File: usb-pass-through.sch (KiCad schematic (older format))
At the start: 7 parts, among them P6 USB_B, P9 USB_A

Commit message: Update with kicad-helpers files
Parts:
- C39: symbol C_Small -> Device:C_Small
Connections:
- wire segments 30 -> 36
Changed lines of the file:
@@
-EESchema Schematic File Version 2
-LIBS:power
-LIBS:device
-LIBS:transistors
-LIBS:conn
-LIBS:linear
-LIBS:regul
-LIBS:74xx
-LIBS:cmos4000
-LIBS:adc-dac
-LIBS:memory
-LIBS:xilinx
-LIBS:microcontrollers
-LIBS:dsp
-LIBS:microchip
-LIBS:analog_switches
-LIBS:motorola
-LIBS:texas
-LIBS:intel
-LIBS:audio
-LIBS:interface
-LIBS:digital-audio
-LIBS:philips
-LIBS:display
-LIBS:cypress
-LIBS:siliconi
-LIBS:opto
-LIBS:atmel
-LIBS:contrib
-LIBS:valves
-LIBS:sci-bots
-LIBS:dropbot_control_board-cache
-EELAYER 25 0
+EESchema Schematic File Version 4
+EELAYER 30 0
 EELAYER END
 $Descr USLetter 11000 8500
@@
 	4850 3450 4750 3450
 Wire Wire Line
-	4750 3250 4750 4150
+	4750 3250 4750 3450
 Wire Wire Line
 	4750 3850 4850 3850
 Connection ~ 4750 3450
 Wire Wire Line
-	5550 3250 5550 4150
+	5550 3250 5550 3450
 Wire Wire Line
 	5550 3850 5450 3850
@@
 $EndComp
 Wire Wire Line
-	4550 3200 4550 3900
+	4550 3200 4550 3650
 $Comp
 L FERRITE FB8
@@
 $EndComp
 Wire Wire Line
-	4550 4200 4550 4400
-$Comp
-L C_Small C39
+	4550 4200 4550 4300
+$Comp
+L Device:C_Small C39
 U 1 1 58BE5178
 P 4250 4300
@@
 	5700 4700 5400 4700
 $Comp
-L GND #PWR025
+L power:GND #PWR025
 U 1 1 5B3C7E87
 P 4800 5100
@@
 	1    0    0    -1
 $EndComp
+Wire Wire Line
+	4750 3450 4750 3850
+Wire Wire Line
+	5550 3450 5550 3850
+Wire Wire Line
+	4750 3850 4750 4150
+Wire Wire Line
+	5550 3850 5550 4150
+Wire Wire Line
+	4550 4300 4550 4400
+Wire Wire Line
+	4550 3650 4550 3900
 $EndSCHEMATC

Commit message: Fix broken symbols and DRC tests
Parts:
- D5: symbol WE-TVS_824015 -> sci-bots:WE-TVS_824015
- FB7, FB8: symbol FERRITE -> sci-bots:FERRITE
- L2: symbol CM_CHOKE -> sci-bots:CM_CHOKE
- P6: symbol USB_B -> Connector:USB_B
- P9: symbol USB_A -> Connector:USB_A
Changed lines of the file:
@@
 CHASIS_GND
 $Comp
-L WE-TVS_824015 D5
+L sci-bots:WE-TVS_824015 D5
 U 1 1 58BAFF99
 P 5150 3650
@@
 $EndComp
 $Comp
-L CM_CHOKE L2
+L sci-bots:CM_CHOKE L2
 U 1 1 58BBE1AE
 P 5150 4300
@@
 	5200 4150 5200 4200
 $Comp
-L FERRITE FB7
+L sci-bots:FERRITE FB7
 U 1 1 58BE3979
 P 4550 4050
@@
 	4550 3200 4550 3650
 $Comp
-L FERRITE FB8
+L sci-bots:FERRITE FB8
 U 1 1 58BE422E
 P 4550 4550
@@
 Wire Wire Line
 	4850 3650 4550 3650
-Text GLabel 5200 4550 2    60   Input ~ 0
-D+
-Text GLabel 5100 4550 0    60   Input ~ 0
-D-
 Wire Wire Line
 	4350 4300 4550 4300
@@
 	3950 4300 4150 4300
 $Comp
-L USB_B P6
+L Connector:USB_B P6
 U 1 1 59320548
 P 5200 2800
@@
 	5700 3650 5450 3650
 $Comp
-L USB_A P9
+L Connector:USB_A P9
 U 1 1 59320AF4
 P 5200 5000
@@
 Wire Wire Line
 	4550 3650 4550 3900
+Text Label 5100 4600 2    60   ~ 0
+D-
+Text Label 5200 4600 0    60   ~ 0
+D+
+$Comp
+L power:PWR_FLAG #FLG0104
+U 1 1 61967CD9
+P 4550 5300
+F 0 "#FLG0104" H 4550 5375 50  0001 C CNN
+F 1 "PWR_FLAG" H 4550 5473 50  0000 C CNN
+F 2 "" H 4550 5300 50  0001 C CNN
+F 3 "~" H 4550 5300 50  0001 C CNN
+	1    4550 5300
+	-1   0    0    1
+$EndComp
+Connection ~ 4550 5300
 $EndSCHEMATC

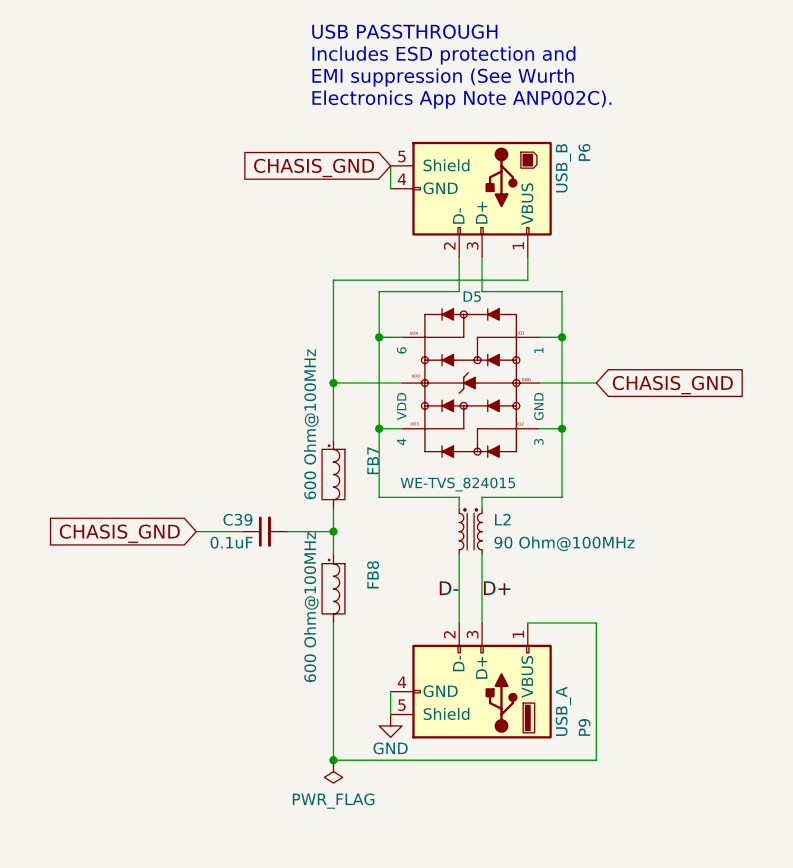
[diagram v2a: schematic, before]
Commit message: Update BOM
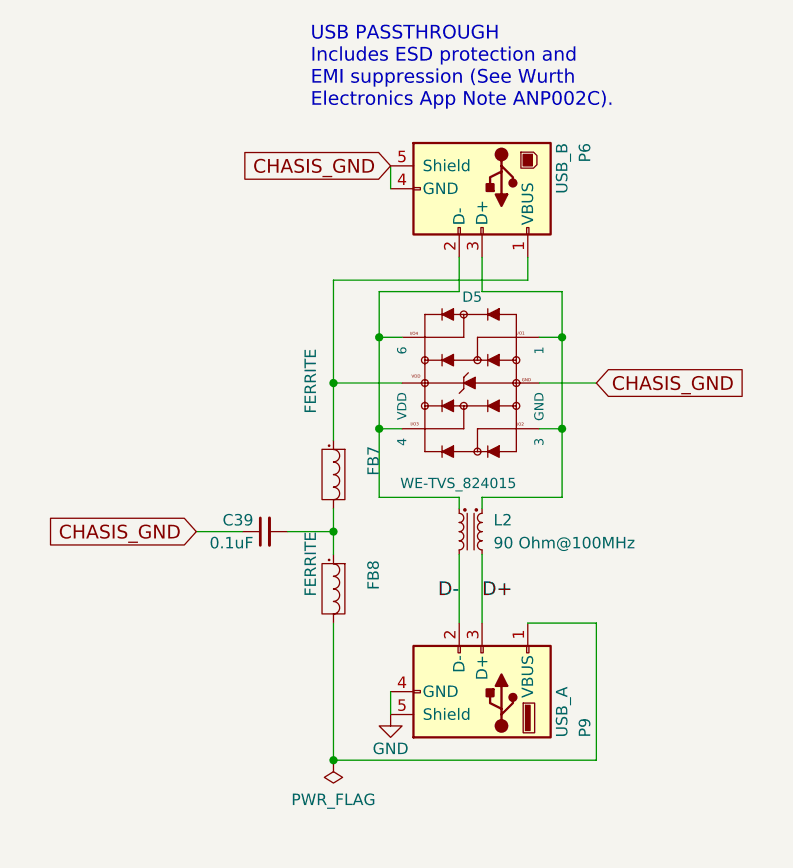
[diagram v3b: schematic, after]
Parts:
- C39: MPN (none) -> CL21B104KBCNNNC; Manufacturer (none) -> Samsung
- D5: MPN (none) -> 824015; Manufacturer (none) -> Würth Elektronik
- FB7, FB8: value 600 Ohm@100MHz -> FERRITE; MPN (none) -> 742792040; Manufacturer (none) -> Würth Elektronik
- L2: MPN (none) -> 744231091; Manufacturer (none) -> Würth Elektronik
- P6: MPN (none) -> 1734346-1; Manufacturer (none) -> TE Connectivity
- P9: MPN (none) -> AU-Y1006; Manufacturer (none) -> ASSMANN WSW Components
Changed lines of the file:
@@
 Comment4 ""
 $EndDescr
+$Comp
+L sci-bots:WE-TVS_824015 D5
+U 1 1 58BAFF99
+P 5150 3650
+F 0 "D5" V 4800 3600 45 0000 L BNN
+F 1 "WE-TVS_824015" V 5615 3450 45 0000 L BNN
+F 2 "Sci-Bots:wurth-WE-TVS_SOT23-6L" H 5180 3800 20 0001 C CNN
+F 3 "" H 5150 3650 60 0000 C CNN
+F 4 "824015" H 4800 3700 50 0001 C CNN "MPN"
+F 5 "Würth Elektronik" H 4800 3700 50 0001 C CNN "Manufacturer"
+F 6 "824015" H 5150 3650 60 0001 C CNN "Mfg_Part_No"
+	1    5150 3650
+	0    -1   1    0
+$EndComp
+$Comp
+L sci-bots:CM_CHOKE L2
+U 1 1 58BBE1AE
+P 5150 4300
+F 0 "L2" H 5250 4350 50 0000 L CNN
+F 1 "90 Ohm@100MHz" H 5250 4250 50 0000 L CNN
+F 2 "Sci-Bots:wurth-WE-CNSW_0805" H 5200 4300 50 0001 C CNN
+F 3 "" H 5200 4300 50 0000 C CNN
+F 4 "744231091" H 5250 4450 50 0001 C CNN "MPN"
+F 5 "Würth Elektronik" H 5250 4450 50 0001 C CNN "Manufacturer"
+F 6 "744231091" H 5150 4300 60 0001 C CNN "Mfg_Part_No"
+	1    5150 4300
+	1    0    0    -1
+$EndComp
+$Comp
+L sci-bots:FERRITE FB7
+U 1 1 58BE3979
+P 4550 4050
+F 0 "FB7" H 4425 4225 50 0000 L CNN
+F 1 "FERRITE" H 4000 3950 50 0000 L CNN
+F 2 "Resistors_SMD:R_0805" H 4550 3950 60 0001 C CNN
+F 3 "" H 4550 3950 60 0000 C CNN
+F 4 "742792040" H 4425 4325 50 0001 C CNN "MPN"
+F 5 "Würth Elektronik" H 4425 4325 50 0001 C CNN "Manufacturer"
+F 6 "742792040" H 4550 4050 60 0001 C CNN "Mfg_Part_No"
+	1    4550 4050
+	0    1    1    0
+$EndComp
+$Comp
+L sci-bots:FERRITE FB8
+U 1 1 58BE422E
+P 4550 4550
+F 0 "FB8" H 4425 4725 50 0000 L CNN
+F 1 "FERRITE" H 4300 4450 50 0000 L CNN
+F 2 "Resistors_SMD:R_0805" H 4550 4450 60 0001 C CNN
+F 3 "" H 4550 4450 60 0000 C CNN
+F 4 "742792040" H 4425 4825 50 0001 C CNN "MPN"
+F 5 "Würth Elektronik" H 4425 4825 50 0001 C CNN "Manufacturer"
+F 6 "742792040" H 4550 4550 60 0001 C CNN "Mfg_Part_No"
+	1    4550 4550
+	0    1    1    0
+$EndComp
+$Comp
+L Device:C_Small C39
+U 1 1 58BE5178
+P 4250 4300
+F 0 "C39" V 4300 4350 50 0000 L CNN
+F 1 "0.1uF" V 4200 4350 50 0000 L CNN
+F 2 "Capacitors_SMD:C_0805" H 4250 4300 50 0001 C CNN
+F 3 "" H 4250 4300 50 0000 C CNN
+F 4 "CL21B104KBCNNNC" H 4300 4450 50 0001 C CNN "MPN"
+F 5 "Samsung" H 4300 4450 50 0001 C CNN "Manufacturer"
+F 6 "CL21B104KBCNNNC" H 4250 4300 60 0001 C CNN "Mfg_Part_No"
+	1    4250 4300
+	0    -1   -1   0
+$EndComp
+$Comp
+L Connector:USB_B P6
+U 1 1 59320548
+P 5200 2800
+F 0 "P6" H 5000 3250 50 0000 L CNN
+F 1 "USB_B" H 5000 3150 50 0000 L CNN
+F 2 "Sci-Bots:1734346-1" H 5350 2750 50 0001 C CNN
+F 3 "" H 5350 2750 50 0001 C CNN
+F 4 "1734346-1" H 5000 3350 50 0001 C CNN "MPN"
+F 5 "TE Connectivity" H 5000 3350 50 0001 C CNN "Manufacturer"
+F 6 "1734346-1" H 5200 2800 60 0001 C CNN "Mfg_Part_No"
+	1    5200 2800
+	0    1    1    0
+$EndComp
+$Comp
+L Connector:USB_A P9
+U 1 1 59320AF4
+P 5200 5000
+F 0 "P9" H 5000 5450 50 0000 L CNN
+F 1 "USB_A" H 5000 5350 50 0000 L CNN
+F 2 "Sci-Bots:AU-Y1006" H 5350 4950 50 0001 C CNN
+F 3 "" H 5350 4950 50 0001 C CNN
+F 4 "AU-Y1006" H 5000 5550 50 0001 C CNN "MPN"
+F 5 "ASSMANN WSW Components" H 5000 5550 50 0001 C CNN "Manufacturer"
+F 6 "AU-Y1006" H 5200 5000 60 0001 C CNN "Mfg_Part_No"
+	1    5200 5000
+	0    1    -1   0
+$EndComp
+$Comp
+L power:GND #PWR025
+U 1 1 5B3C7E87
+P 4800 5100
+F 0 "#PWR025" H 4800 4850 50 0001 C CNN
+F 1 "GND" H 4800 4950 50 0000 C CNN
+F 2 "" H 4800 5100 50 0001 C CNN
+F 3 "" H 4800 5100 50 0001 C CNN
+	1    4800 5100
+	1    0    0    -1
+$EndComp
+$Comp
+L power:PWR_FLAG #FLG0104
+U 1 1 61967CD9
+P 4550 5300
+F 0 "#FLG0104" H 4550 5375 50 0001 C CNN
+F 1 "PWR_FLAG" H 4550 5473 50 0000 C CNN
+F 2 "" H 4550 5300 50 0001 C CNN
+F 3 "~" H 4550 5300 50 0001 C CNN
+	1    4550 5300
+	-1   0    0    1
+$EndComp
 Text Notes 4450 2450 0    60   ~ 0
 USB PASSTHROUGH\nIncludes ESD protection and\nEMI suppression (See Wurth\nElectronics App Note ANP002C).
 Text GLabel 5700 3650 2    60   Input ~ 0
 CHASIS_GND
-$Comp
-L sci-bots:WE-TVS_824015 D5
-U 1 1 58BAFF99
-P 5150 3650
-F 0 "D5" V 4800 3600 45  0000 L BNN
-F 1 "WE-TVS_824015" V 5615 3450 45  0000 L BNN
-F 2 "Sci-Bots:wurth-WE-TVS_SOT23-6L" H 5180 3800 20  0001 C CNN
-F 3 "" H 5150 3650 60  0000 C CNN
-F 4 "824015" H 5150 3650 60  0001 C CNN "Mfg_Part_No"
-	1    5150 3650
-	0    -1   1    0
-$EndComp
-$Comp
-L sci-bots:CM_CHOKE L2
-U 1 1 58BBE1AE
-P 5150 4300
-F 0 "L2" H 5250 4350 50  0000 L CNN
-F 1 "90 Ohm@100MHz" H 5250 4250 50  0000 L CNN
-F 2 "Sci-Bots:wurth-WE-CNSW_0805" H 5200 4300 50  0001 C CNN
-F 3 "" H 5200 4300 50  0000 C CNN
-F 4 "744231091" H 5150 4300 60  0001 C CNN "Mfg_Part_No"
-	1    5150 4300
-	1    0    0    -1
-$EndComp
-Wire Wire Line
-	5100 3100 5100 3250
-Wire Wire Line
-	5100 3250 4750 3250
-Wire Wire Line
-	5200 3100 5200 3250
-Wire Wire Line
-	5200 3250 5550 3250
-Wire Wire Line
-	4850 3450 4750 3450
-Wire Wire Line
-	4750 3250 4750 3450
-Wire Wire Line
-	4750 3850 4850 3850
-Connection ~ 4750 3450
-Wire Wire Line
-	5550 3250 5550 3450
-Wire Wire Line
-	5550 3850 5450 3850
-Wire Wire Line
-	5450 3450 5550 3450
-Connection ~ 5550 3450
-Connection ~ 4750 3850
-Connection ~ 5550 3850
-Wire Wire Line
-	4750 4150 5100 4150
-Wire Wire Line
-	5550 4150 5200 4150
-Wire Wire Line
-	5100 4150 5100 4200
-Wire Wire Line
-	5200 4150 5200 4200
-$Comp
-L sci-bots:FERRITE FB7
-U 1 1 58BE3979
-P 4550 4050
-F 0 "FB7" H 4425 4225 50  0000 L CNN
-F 1 "600 Ohm@100MHz" H 4000 3950 50  0000 L CNN
-F 2 "Resistors_SMD:R_0805" H 4550 3950 60  0001 C CNN
-F 3 "" H 4550 3950 60  0000 C CNN
-F 4 "742792040" H 4550 4050 60  0001 C CNN "Mfg_Part_No"
-	1    4550 4050
-	0    1    1    0
-$EndComp
-Wire Wire Line
-	4550 3200 4550 3650
-$Comp
-L sci-bots:FERRITE FB8
-U 1 1 58BE422E
-P 4550 4550
-F 0 "FB8" H 4425 4725 50  0000 L CNN
-F 1 "600 Ohm@100MHz" H 4300 4450 50  0000 L CNN
-F 2 "Resistors_SMD:R_0805" H 4550 4450 60  0001 C CNN
-F 3 "" H 4550 4450 60  0000 C CNN
-F 4 "742792040" H 4550 4550 60  0001 C CNN "Mfg_Part_No"
-	1    4550 4550
-	0    1    1    0
-$EndComp
-Wire Wire Line
-	4550 4200 4550 4300
-$Comp
-L Device:C_Small C39
-U 1 1 58BE5178
-P 4250 4300
-F 0 "C39" V 4300 4350 50  0000 L CNN
-F 1 "0.1uF" V 4200 4350 50  0000 L CNN
-F 2 "Capacitors_SMD:C_0805" H 4250 4300 50  0001 C CNN
-F 3 "" H 4250 4300 50  0000 C CNN
-F 4 "CL21B104KBCNNNC" H 4250 4300 60  0001 C CNN "Mfg_Part_No"
-	1    4250 4300
-	0    -1   -1   0
-$EndComp
-Connection ~ 4550 4300
-Connection ~ 4550 3650
-Wire Wire Line
-	4850 3650 4550 3650
-Wire Wire Line
-	4350 4300 4550 4300
 Text GLabel 3950 4300 0    60   Input ~ 0
 CHASIS_GND
-Wire Wire Line
-	3950 4300 4150 4300
-$Comp
-L Connector:USB_B P6
-U 1 1 59320548
-P 5200 2800
-F 0 "P6" H 5000 3250 50  0000 L CNN
-F 1 "USB_B" H 5000 3150 50  0000 L CNN
-F 2 "Sci-Bots:1734346-1" H 5350 2750 50  0001 C CNN
-F 3 "" H 5350 2750 50  0001 C CNN
-F 4 "1734346-1" H 5200 2800 60  0001 C CNN "Mfg_Part_No"
-	1    5200 2800
-	0    1    1    0
-$EndComp
-Wire Wire Line
-	4550 3200 5400 3200
-Wire Wire Line
-	5400 3200 5400 3100
-Wire Wire Line
-	5700 3650 5450 3650
-$Comp
-L Connector:USB_A P9
-U 1 1 59320AF4
-P 5200 5000
-F 0 "P9" H 5000 5450 50  0000 L CNN
-F 1 "USB_A" H 5000 5350 50  0000 L CNN
-F 2 "Sci-Bots:AU-Y1006" H 5350 4950 50  0001 C CNN
-F 3 "" H 5350 4950 50  0001 C CNN
-F 4 "AU-Y1006" H 5200 5000 60  0001 C CNN "Mfg_Part_No"
-	1    5200 5000
-	0    1    -1   0
-$EndComp
 Text GLabel 4800 2700 0    60   Input ~ 0
 CHASIS_GND
-Wire Wire Line
-	4800 2800 4800 2700
-Wire Wire Line
-	5100 4700 5100 4400
-Wire Wire Line
-	5200 4400 5200 4700
-Wire Wire Line
-	4800 5000 4800 5100
-Wire Wire Line
-	4550 4700 4550 5300
-Wire Wire Line
-	4550 5300 5700 5300
-Wire Wire Line
-	5700 5300 5700 4700
-Wire Wire Line
-	5700 4700 5400 4700
-$Comp
-L power:GND #PWR025
-U 1 1 5B3C7E87
-P 4800 5100
-F 0 "#PWR025" H 4800 4850 50  0001 C CNN
-F 1 "GND" H 4800 4950 50  0000 C CNN
-F 2 "" H 4800 5100 50  0001 C CNN
-F 3 "" H 4800 5100 50  0001 C CNN
-	1    4800 5100
-	1    0    0    -1
-$EndComp
-Wire Wire Line
-	4750 3450 4750 3850
-Wire Wire Line
-	5550 3450 5550 3850
-Wire Wire Line
-	4750 3850 4750 4150
-Wire Wire Line
-	5550 3850 5550 4150
-Wire Wire Line
-	4550 4300 4550 4400
-Wire Wire Line
-	4550 3650 4550 3900
 Text Label 5100 4600 2    60   ~ 0
 D-
 Text Label 5200 4600 0    60   ~ 0
 D+
-$Comp
-L power:PWR_FLAG #FLG0104
-U 1 1 61967CD9
-P 4550 5300
-F 0 "#FLG0104" H 4550 5375 50  0001 C CNN
-F 1 "PWR_FLAG" H 4550 5473 50  0000 C CNN
-F 2 "" H 4550 5300 50  0001 C CNN
-F 3 "~" H 4550 5300 50  0001 C CNN
-	1    4550 5300
-	-1   0    0    1
-$EndComp
+Wire Wire Line
+	5100 3100 5100 3250
+Wire Wire Line
+	5100 3250 4750 3250
+Wire Wire Line
+	5200 3100 5200 3250
+Wire Wire Line
+	5200 3250 5550 3250
+Wire Wire Line
+	4850 3450 4750 3450
+Wire Wire Line
+	4750 3250 4750 3450
+Wire Wire Line
+	4750 3850 4850 3850
+Wire Wire Line
+	5550 3250 5550 3450
+Wire Wire Line
+	5550 3850 5450 3850
+Wire Wire Line
+	5450 3450 5550 3450
+Wire Wire Line
+	4750 4150 5100 4150
+Wire Wire Line
+	5550 4150 5200 4150
+Wire Wire Line
+	5100 4150 5100 4200
+Wire Wire Line
+	5200 4150 5200 4200
+Wire Wire Line
+	4550 3200 4550 3650
+Wire Wire Line
+	4550 4200 4550 4300
+Wire Wire Line
+	4850 3650 4550 3650
+Wire Wire Line
+	4350 4300 4550 4300
+Wire Wire Line
+	3950 4300 4150 4300
+Wire Wire Line
+	4550 3200 5400 3200
+Wire Wire Line
+	5400 3200 5400 3100
+Wire Wire Line
+	5700 3650 5450 3650
+Wire Wire Line
+	4800 2800 4800 2700
+Wire Wire Line
+	5100 4700 5100 4400
+Wire Wire Line
+	5200 4400 5200 4700
+Wire Wire Line
+	4800 5000 4800 5100
+Wire Wire Line
+	4550 4700 4550 5300
+Wire Wire Line
+	4550 5300 5700 5300
+Wire Wire Line
+	5700 5300 5700 4700
+Wire Wire Line
+	5700 4700 5400 4700
+Wire Wire Line
+	4750 3450 4750 3850
+Wire Wire Line
+	5550 3450 5550 3850
+Wire Wire Line
+	4750 3850 4750 4150
+Wire Wire Line
+	5550 3850 5550 4150
+Wire Wire Line
+	4550 4300 4550 4400
+Wire Wire Line
+	4550 3650 4550 3900
+Connection ~ 4750 3450
+Connection ~ 5550 3450
+Connection ~ 4750 3850
+Connection ~ 5550 3850
+Connection ~ 4550 4300
+Connection ~ 4550 3650
 Connection ~ 4550 5300
 $EndSCHEMATC

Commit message: Remove "Mfg_Part_No" field (replaced by  "MPN")
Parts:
- C39: Mfg_Part_No CL21B104KBCNNNC -> (none)
- D5: Mfg_Part_No 824015 -> (none)
- FB7, FB8: Mfg_Part_No 742792040 -> (none)
- L2: Mfg_Part_No 744231091 -> (none)
- P6: Mfg_Part_No 1734346-1 -> (none)
- P9: Mfg_Part_No AU-Y1006 -> (none)
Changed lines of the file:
@@
 F 4 "824015" H 4800 3700 50 0001 C CNN "MPN"
 F 5 "Würth Elektronik" H 4800 3700 50 0001 C CNN "Manufacturer"
-F 6 "824015" H 5150 3650 60 0001 C CNN "Mfg_Part_No"
 	1    5150 3650
 	0    -1   1    0
@@
 F 4 "744231091" H 5250 4450 50 0001 C CNN "MPN"
 F 5 "Würth Elektronik" H 5250 4450 50 0001 C CNN "Manufacturer"
-F 6 "744231091" H 5150 4300 60 0001 C CNN "Mfg_Part_No"
 	1    5150 4300
 	1    0    0    -1
@@
 F 4 "742792040" H 4425 4325 50 0001 C CNN "MPN"
 F 5 "Würth Elektronik" H 4425 4325 50 0001 C CNN "Manufacturer"
-F 6 "742792040" H 4550 4050 60 0001 C CNN "Mfg_Part_No"
 	1    4550 4050
 	0    1    1    0
@@
 F 4 "742792040" H 4425 4825 50 0001 C CNN "MPN"
 F 5 "Würth Elektronik" H 4425 4825 50 0001 C CNN "Manufacturer"
-F 6 "742792040" H 4550 4550 60 0001 C CNN "Mfg_Part_No"
 	1    4550 4550
 	0    1    1    0
@@
 F 4 "CL21B104KBCNNNC" H 4300 4450 50 0001 C CNN "MPN"
 F 5 "Samsung" H 4300 4450 50 0001 C CNN "Manufacturer"
-F 6 "CL21B104KBCNNNC" H 4250 4300 60 0001 C CNN "Mfg_Part_No"
 	1    4250 4300
 	0    -1   -1   0
@@
 F 4 "1734346-1" H 5000 3350 50 0001 C CNN "MPN"
 F 5 "TE Connectivity" H 5000 3350 50 0001 C CNN "Manufacturer"
-F 6 "1734346-1" H 5200 2800 60 0001 C CNN "Mfg_Part_No"
 	1    5200 2800
 	0    1    1    0
@@
 F 4 "AU-Y1006" H 5000 5550 50 0001 C CNN "MPN"
 F 5 "ASSMANN WSW Components" H 5000 5550 50 0001 C CNN "Manufacturer"
-F 6 "AU-Y1006" H 5200 5000 60 0001 C CNN "Mfg_Part_No"
 	1    5200 5000
 	0    1    -1   0
